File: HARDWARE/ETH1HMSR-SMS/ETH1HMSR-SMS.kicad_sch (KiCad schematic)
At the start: 5 parts

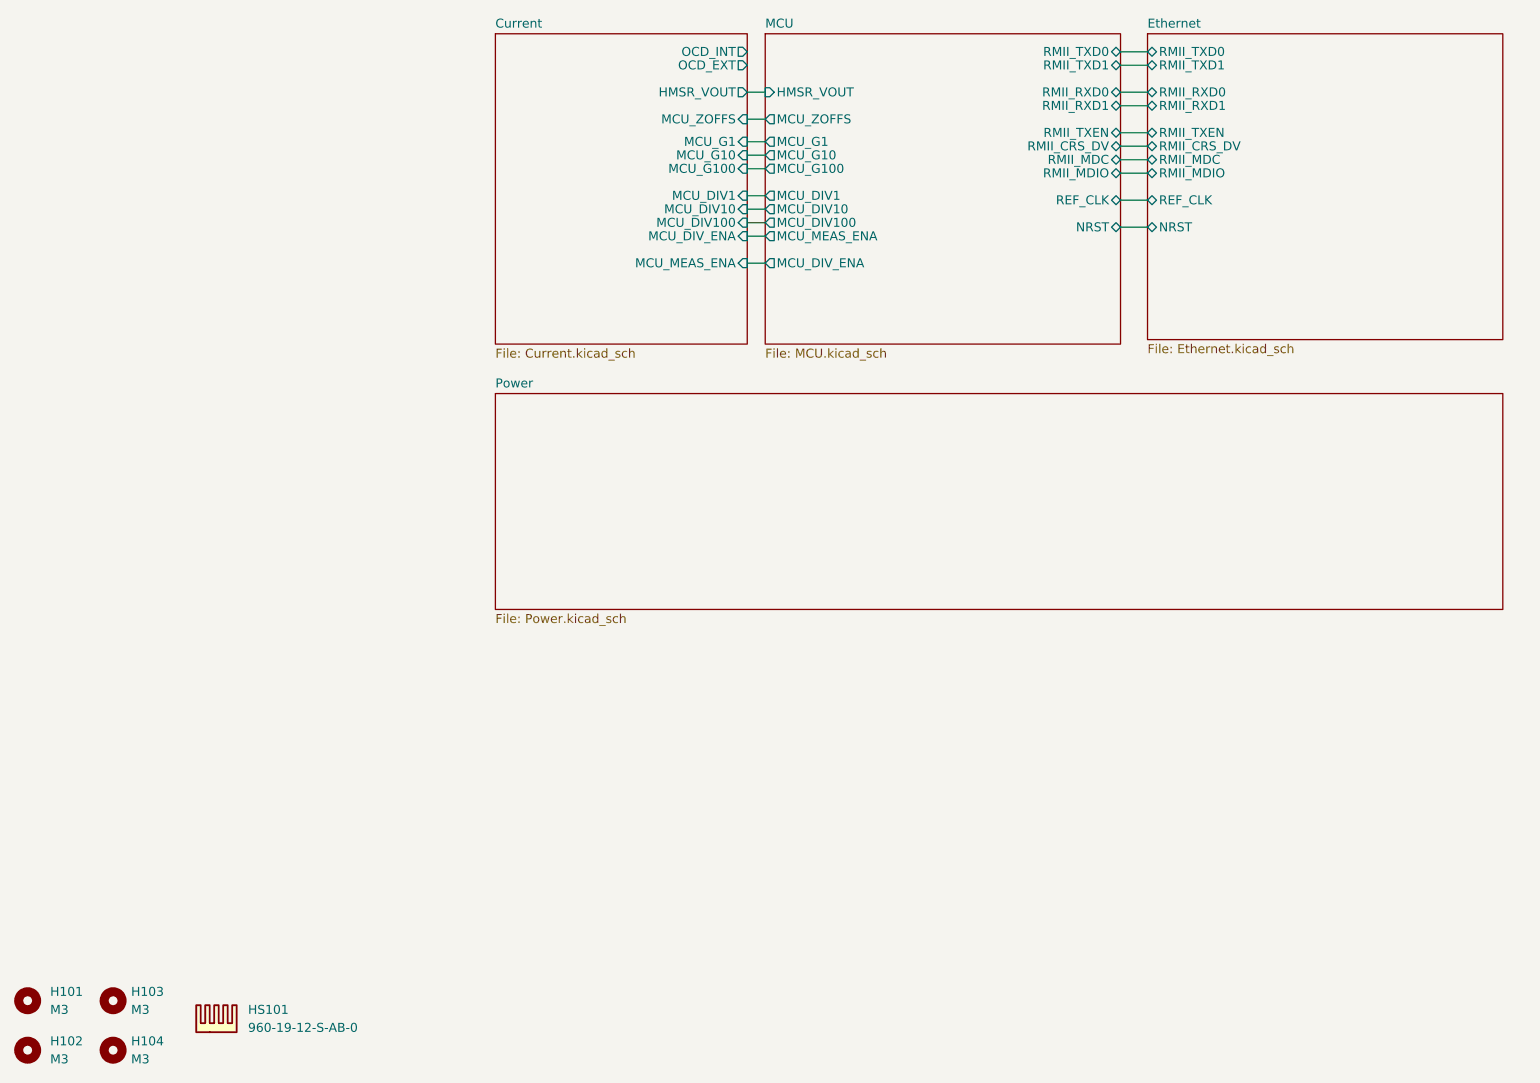
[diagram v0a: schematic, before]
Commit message: Development
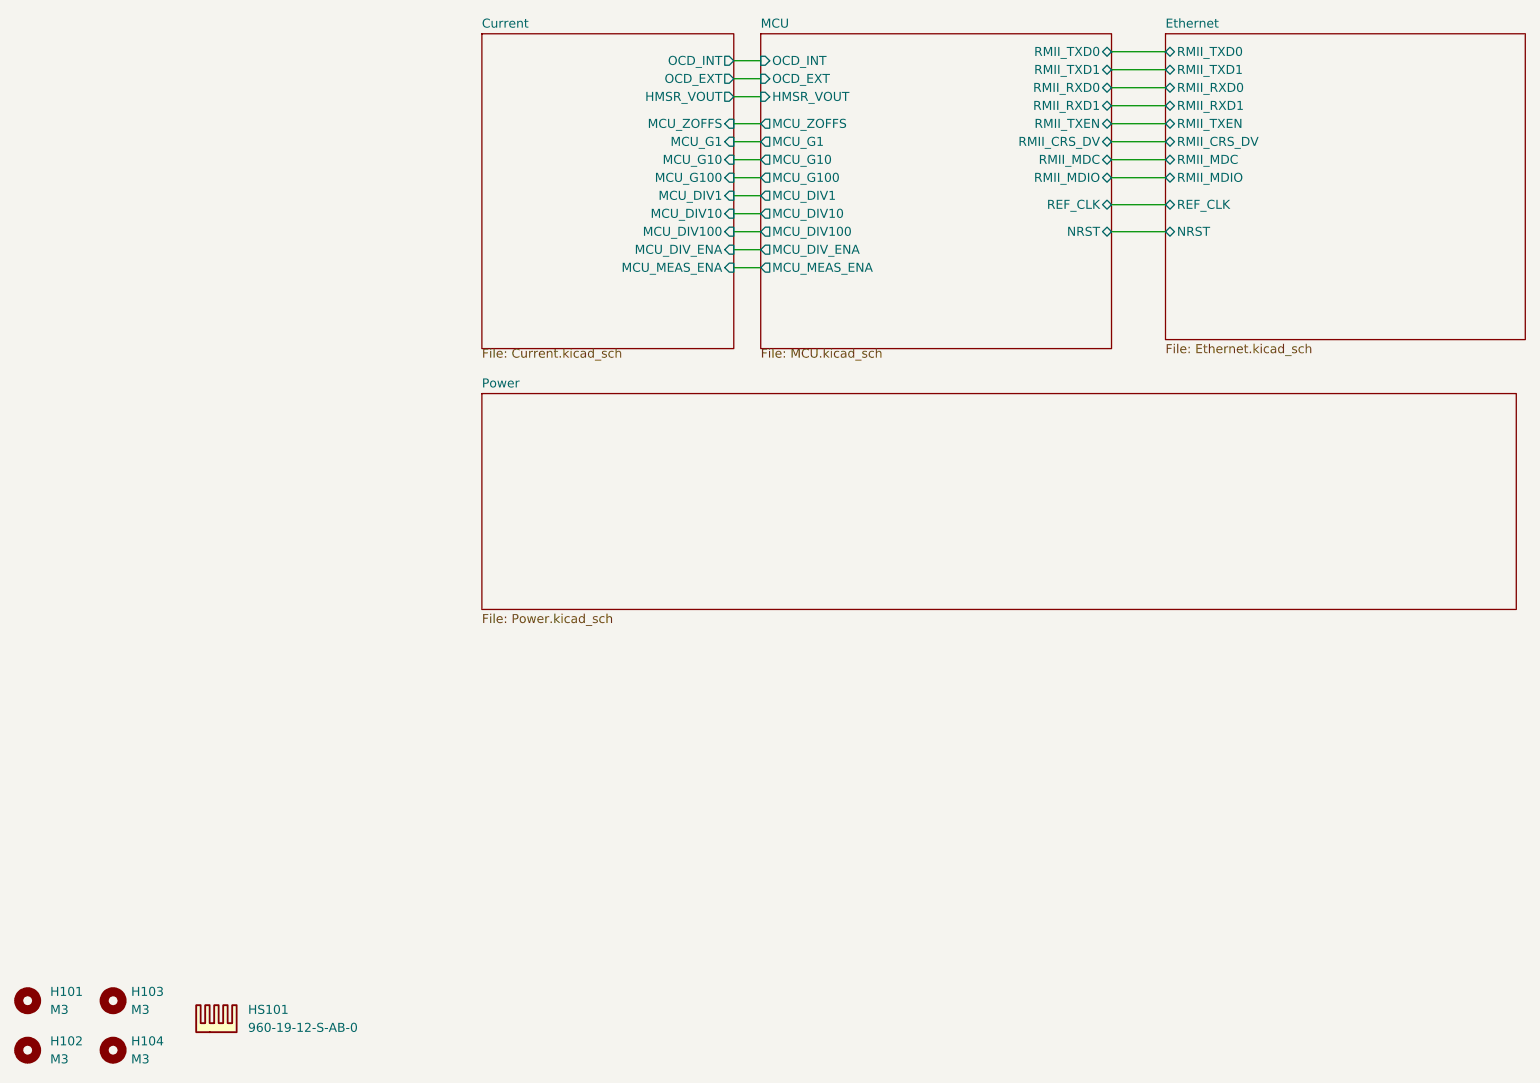
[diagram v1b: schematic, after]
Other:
- sheet MCU ports: added OCD_EXT, OCD_INT; removed none
